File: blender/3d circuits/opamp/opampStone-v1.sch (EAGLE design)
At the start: 13 parts, among them Q2 IRLML0060, Q3 IRLML0060, Q4 IRLML0060, Q5 IRLML0060

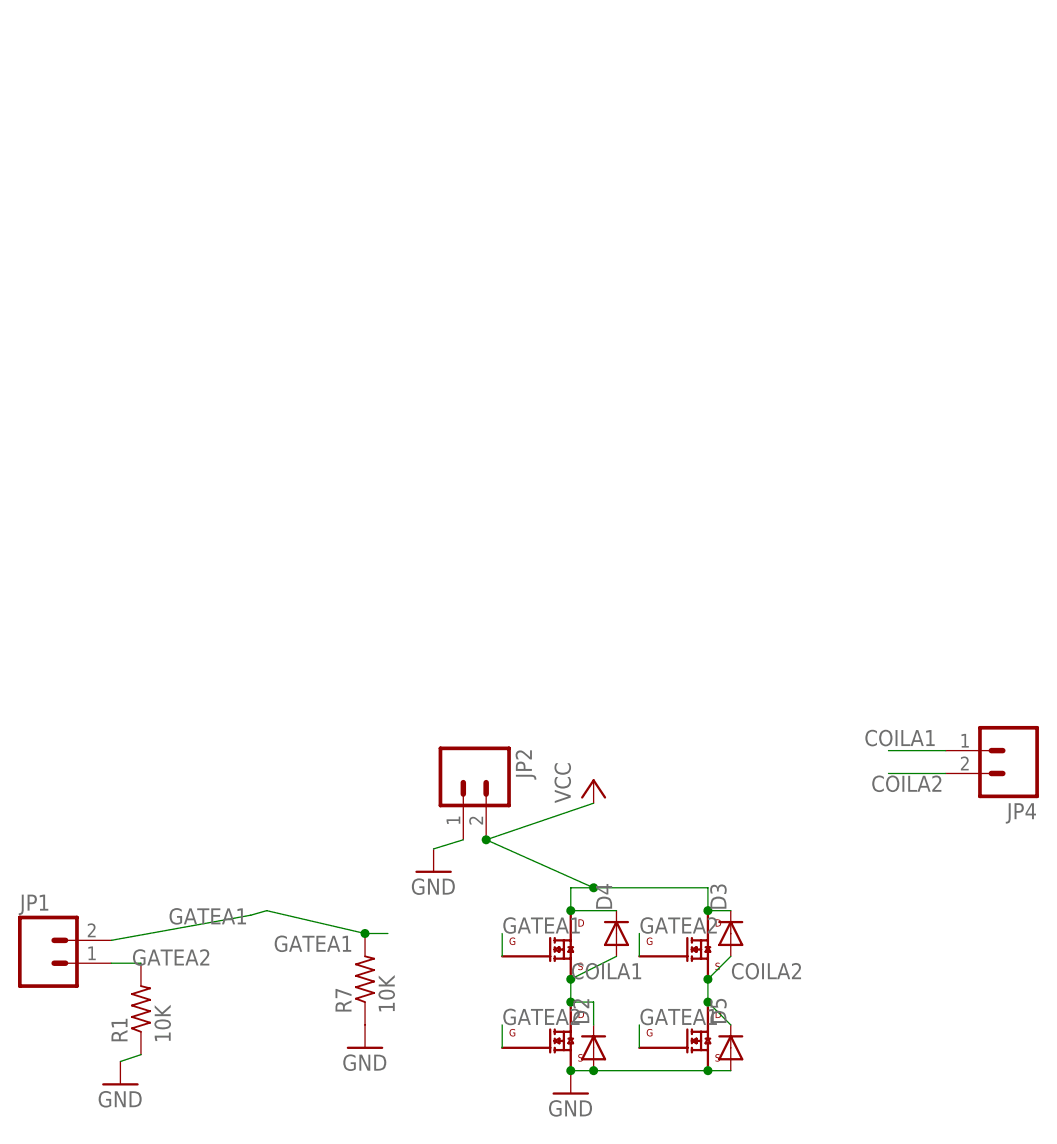
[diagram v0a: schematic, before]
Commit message: 3d circuit design
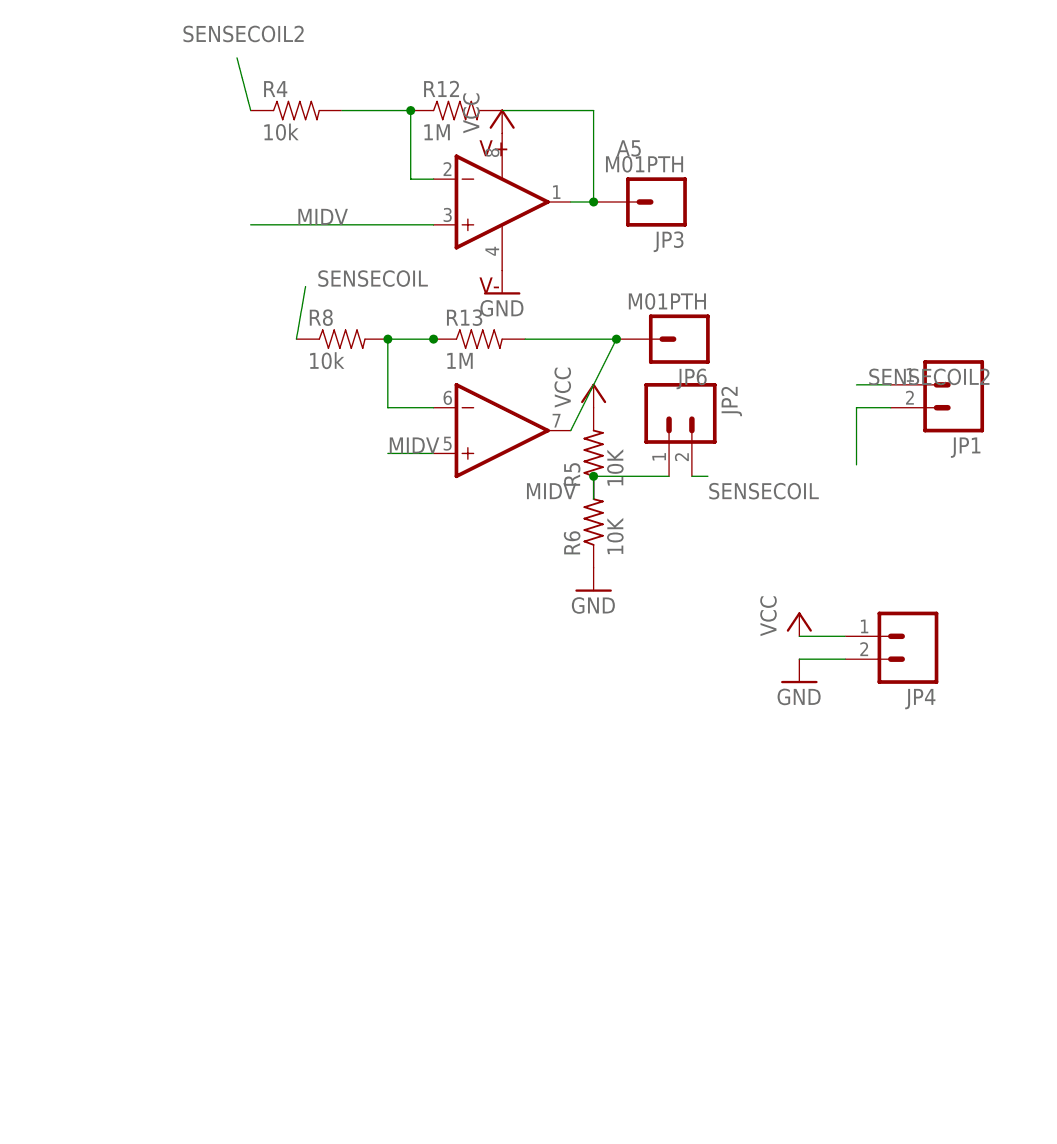
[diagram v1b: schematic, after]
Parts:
- removed D2, D3, D4, D5: (no value), diode:DIODE-DO-214AC
- removed Q2, Q3, Q4, Q5: IRLML0060, spietz-library:IRLML0060
- removed R1, R7: 10K, resistor:R-US_R0603
- added JP3, JP6: M01PTH, SparkFun-Connectors:M01PTH
- added R12, R13: 1M, SparkFun-Passives:RESISTOR0805-RES
- added R4, R8: 10k, SparkFun-Resistors:RESISTOR0603
- added R5, R6: 10K, resistor:R-US_R0603
- added U2: MCP6242, spietz-library:MCP6242
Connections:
- removed net COILA1: D2.C, D4.A, JP4.1, Q2.DRAIN, Q4.SOURCE
- removed net COILA2: D3.A, D5.C, JP4.2, Q3.SOURCE, Q5.DRAIN
- removed net GATEA1: JP1.2, Q4.GATE, Q5.GATE, R7.2
- removed net GATEA2: JP1.1, Q2.GATE, Q3.GATE, R1.2
- new net A4: JP6.1, R13.2, U2.OUTB
- new net A5: JP3.1, R12.2, U2.OUTA
- new net MIDV: JP1.2, JP2.1, R5.1, R6.2, U2.+INA, U2.+INB
- new net N$13: R12.1, R4.2, U2.-INA
- new net N$15: R13.1, R8.2, U2.-INB
- new net SENSECOIL: JP2.2, R8.1
- new net SENSECOIL2: JP1.1, R4.1
- net GND: now also JP4.2, R6.1, U2.V-; no longer D2.A, D5.A, JP2.1, Q2.SOURCE, Q5.SOURCE, R1.1, R7.1
- net VCC: now also JP4.1, R5.2, U2.V+; no longer D3.C, D4.C, JP2.2, Q3.DRAIN, Q4.DRAIN
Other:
- moved on the sheet: JP1, JP2, JP4
